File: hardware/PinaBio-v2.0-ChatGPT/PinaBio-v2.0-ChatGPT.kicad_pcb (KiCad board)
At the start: 4 copper layers, 96 x 96 mm, 93 parts, among them J1 USB-C USB2.0 16P, J2 LiPo 1S protected + NTC, J3 AD8232 external module, J4 GSR, J5 RESP_T, J6 RESP_A, J7 GY-30102 external, J8 CJMCU-30205 external, J9 DEBUG UART, SW1 ON/OFF DPDT, SW2 BOOT, SW3 RESET, U1 USBLC6-2SC6, U2 BQ24074RGT, U3 TPS63070RNM, U4 TLV75530PDBVR, U5 ESP32-S3-MINI-1U-N8, U6 ADS122C04IPW, U7 ADS122C04IPW, U8 MCP6004

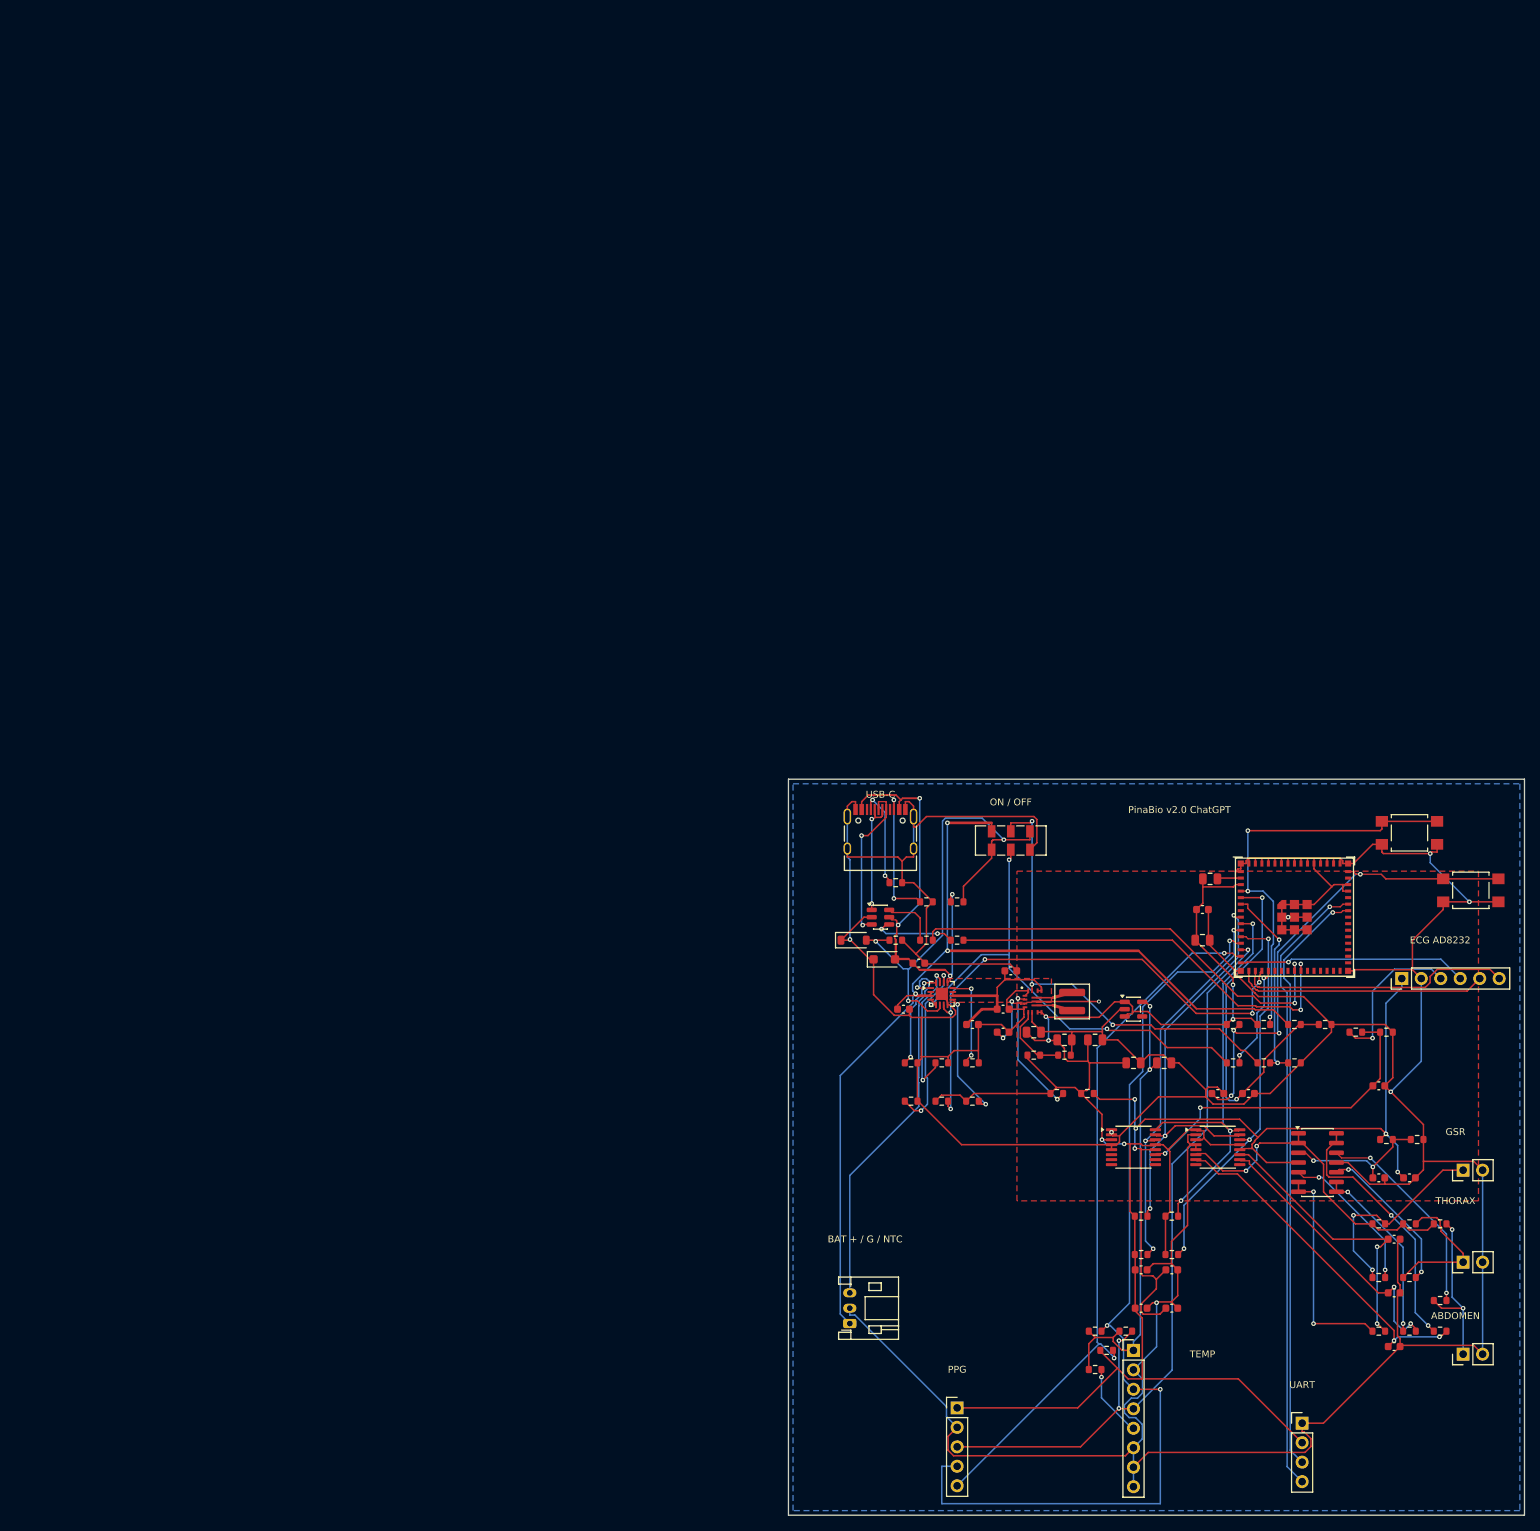
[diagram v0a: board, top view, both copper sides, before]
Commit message: Complete PinaBio Paca v2 ChatGPT KiCad 9 prototype
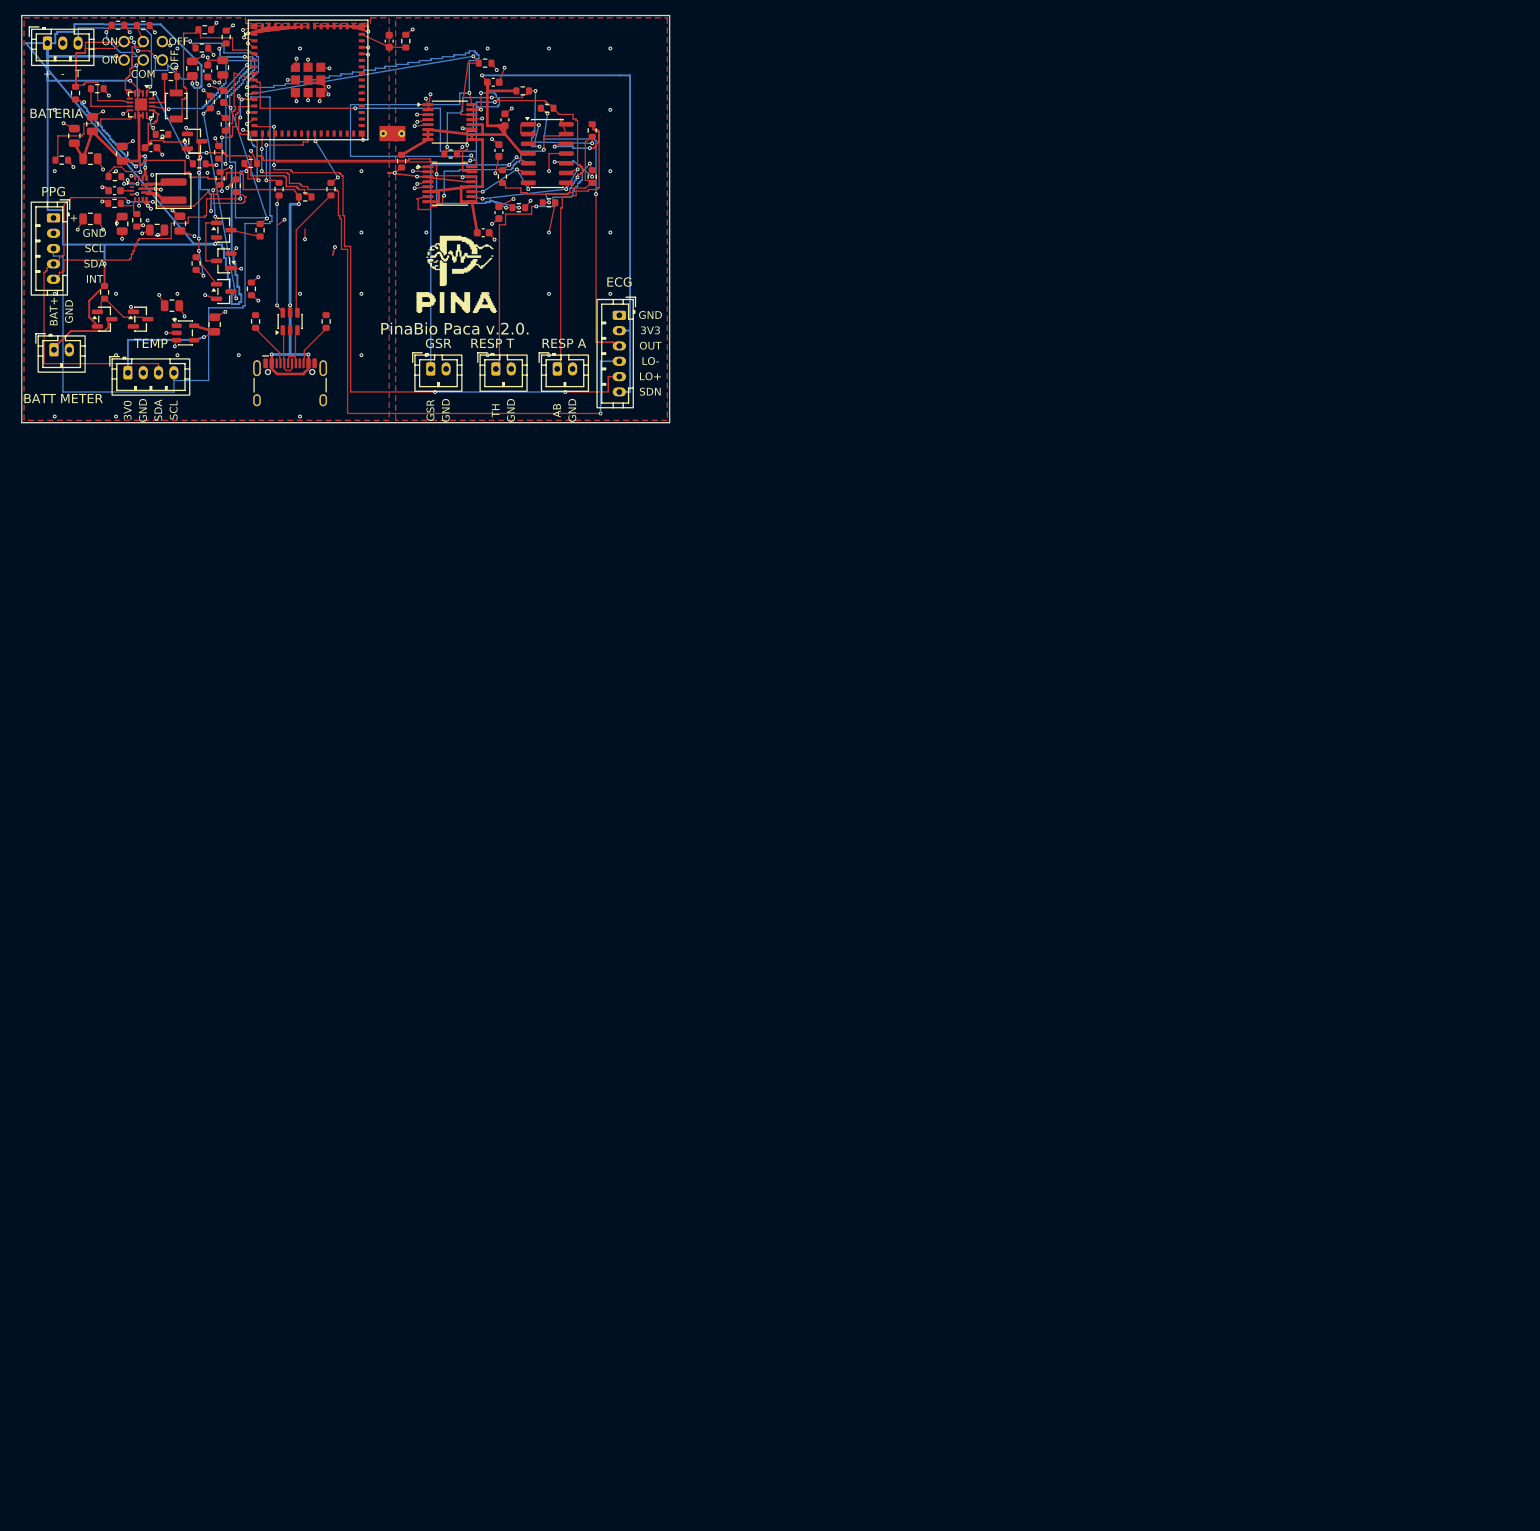
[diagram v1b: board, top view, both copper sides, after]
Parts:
- removed C23: 100nF X7R, Capacitor_SMD:C_0603_1608Metric
- removed C24, C25, C26: 1uF X7R, Capacitor_SMD:C_0603_1608Metric
- removed D2: SMF5.0A, Diode_SMD:D_SOD-123F
- removed R41, R42: 4.7k, Resistor_SMD:R_0603_1608Metric
- removed R43, R44: 10k, Resistor_SMD:R_0603_1608Metric
- removed SW3: RESET, Button_Switch_SMD:SW_SPST_TL3305A
- added NT1: GND_TIE, PinaCursor:GndTie_2mm, F.Cu at (48.3, 15.8)
- added Q1: BSS84, Package_TO_SOT_SMD:SOT-23, F.Cu at (26.3, 28.4)
- added Q2: BSS138, Package_TO_SOT_SMD:SOT-23, F.Cu at (26.3, 32.4)
- added Q3: BSS138, Package_TO_SOT_SMD:SOT-23, F.Cu at (26.3, 36.4)
- added Q4: BSS84, Package_TO_SOT_SMD:SOT-23, F.Cu at (10.8, 40.0)
- added Q5: BSS138, Package_TO_SOT_SMD:SOT-23, F.Cu at (15.5, 40.0)
- C1: value 1uF 16V X7R -> 4.7uF
- C10: value 2.2uF 6.3V X7R -> 10uF
- C11: value 2.2uF 6.3V X7R -> 100nF; footprint Capacitor_SMD:C_0805_2012Metric -> Capacitor_SMD:C_0603_1608Metric
- C12: value 1uF X7R -> 2.2uF; footprint Capacitor_SMD:C_0603_1608Metric -> Capacitor_SMD:C_0805_2012Metric
- C13: value 100nF X7R -> 2.2uF; footprint Capacitor_SMD:C_0603_1608Metric -> Capacitor_SMD:C_0805_2012Metric
- C14: value 10uF 6.3V X7R -> 100nF; footprint Capacitor_SMD:C_0805_2012Metric -> Capacitor_SMD:C_0603_1608Metric
- C15: value 100nF X7R -> 1uF
- C16: value 10uF 6.3V X7R -> 10uF
- C17, C18, C19, C20: value 100nF X7R -> 100nF
- C2: value 4.7uF 10V X7R -> 10uF; footprint Capacitor_SMD:C_0603_1608Metric -> Capacitor_SMD:C_0805_2012Metric
- C21: value 33nF X7R -> 100nF
- C22: value 1uF X7R -> 100nF
- C3, C4, C5: value 10uF 10V X7R -> 10uF; footprint Capacitor_SMD:C_0603_1608Metric -> Capacitor_SMD:C_0805_2012Metric
- C6: value 100nF X7R -> 10uF; footprint Capacitor_SMD:C_0603_1608Metric -> Capacitor_SMD:C_0805_2012Metric
- C7, C8, C9: value 22uF 6.3V X7R -> 22uF
- D1: value BZT52C3V3 -> BZX84-C3V6; footprint Diode_SMD:D_SOD-123 -> Package_TO_SOT_SMD:SOT-23
- J1: value USB-C USB2.0 16P -> USB-C; footprint Connector_USB:USB_C_Receptacle_HRO_TYPE-C-31-M-12 -> Connector_USB:USB_C_Receptacle_HCTL_HC-TYPE-C-16P-01A
- J2: value LiPo 1S protected + NTC -> J_BATT; footprint Connector_JST:JST_PH_S3B-PH-K_1x03_P2.00mm_Horizontal -> Connector_JST:JST_PH_B3B-PH-K_1x03_P2.00mm_Vertical
- J3: value AD8232 external module -> J_ECG; footprint Connector_PinHeader_2.54mm:PinHeader_1x06_P2.54mm_Vertical -> Connector_JST:JST_PH_B6B-PH-K_1x06_P2.00mm_Vertical
- J4: value GSR -> J_PPG; footprint Connector_PinHeader_2.54mm:PinHeader_1x02_P2.54mm_Vertical -> Connector_JST:JST_PH_B5B-PH-K_1x05_P2.00mm_Vertical
- J5: value RESP_T -> J_TEMP; footprint Connector_PinHeader_2.54mm:PinHeader_1x02_P2.54mm_Vertical -> Connector_JST:JST_PH_B4B-PH-K_1x04_P2.00mm_Vertical
- J6: value RESP_A -> J_GSR; footprint Connector_PinHeader_2.54mm:PinHeader_1x02_P2.54mm_Vertical -> Connector_JST:JST_PH_B2B-PH-K_1x02_P2.00mm_Vertical
- J7: value GY-30102 external -> J_RESP_T; footprint Connector_PinHeader_2.54mm:PinHeader_1x05_P2.54mm_Vertical -> Connector_JST:JST_PH_B2B-PH-K_1x02_P2.00mm_Vertical
- J8: value CJMCU-30205 external -> J_RESP_A; footprint Connector_PinHeader_2.54mm:PinHeader_1x08_P2.54mm_Vertical -> Connector_JST:JST_PH_B2B-PH-K_1x02_P2.00mm_Vertical
- J9: value DEBUG UART -> J_BATT_METER; footprint Connector_PinHeader_2.54mm:PinHeader_1x04_P2.54mm_Vertical -> Connector_JST:JST_PH_B2B-PH-K_1x02_P2.00mm_Vertical
- L1: value XAL4020-152MEC 1.5uH -> 1.5uH
- R1, R2: value 5.1k 1% -> 5.1k
- R10: value 46.4k 1% -> 100k
- R11, R12: value 10k -> 100k
- R15: value 10k -> 0
- R16: value 0R -> 1M
- R17: value 10k -> 1M
- R18: value 10k -> 330k
- R19: value 1M 1% -> 100k
- R20: value 330k 1% -> 100k
- R22: value 100k -> 10k
- R23: value 100k -> 4.7k
- R24: value 2.2k -> 4.7k
- R25: value 2.2k -> 10k
- R28: value 33.2k 1% -> 56k 1%
- R29: value 47.5k 1% -> 10k 1%
- R3: value 100k 1% -> 0
- R30: value 56k 1% -> 100k
- R31: value 10k 1% -> 100k
- R32: value 100k 1% -> 100k
- R33: value 100k 1% -> 33.2k 1%
- R34: value 100k 1% -> 47.5k 1%
- R35, R36: value 100k 1% -> 22
- R37: value 100k 1% -> 46.4k 1%
- R38: value 10k 1% -> 10k
- R4: value 150k 1% -> 10.0k
- R40: value 10k 1% -> 1M
- R5: value 22R -> 15.0k
- R6: value 22R -> 2.94k 1%
- R7: value 3.00k 1% -> 2.94k 1%
- R8: value 3.00k 1% -> 2.2k
- R9: value 1.50k 1% -> 100k
- SW1: value ON/OFF DPDT -> DPDT caja; footprint Button_Switch_SMD:SW_DPDT_CK_JS202011JCQN -> PinaCursor:SW_ext_6pad
- SW2: footprint Button_Switch_SMD:SW_SPST_TL3305A -> Button_Switch_SMD:SW_SPST_B3U-1000P
- U2: value BQ24074RGT -> BQ24074
- U3: value TPS63070RNM -> TPS63070; footprint PinaBio-ChatGPT:TPS63070_RNM0015A -> PinaCursor:TPS63070RNM
- U5: footprint PinaBio-ChatGPT:ESP32-S3-MINI-1U -> RF_Module:ESP32-S2-MINI-1U
- U6, U7: value ADS122C04IPW -> ADS122C04
- moved R38 228.6 mm to (23.9, 2.25)
- moved R39 226.3 mm to (12.2, 21.4)
- moved J4 221.9 mm to (4.14, 26.8), turned to -90 degrees
- moved R40 220.7 mm to (10.8, 36.5), turned to 90 degrees
- moved R37 218.7 mm to (25.7, 18.2), turned to 90 degrees
- moved J9 214.7 mm to (4.20, 44.0)
- moved J5 209.3 mm to (13.8, 47.0), turned to 0 degrees
- moved R35 201.8 mm to (33.6, 23.0), turned to 90 degrees
- moved R36 199.9 mm to (40.3, 23.0), turned to 90 degrees
- moved C17 198.2 mm to (24.3, 7.63), turned to 90 degrees
- moved J2 197.1 mm to (3.35, 4.00), turned to 0 degrees
- moved R24 195.5 mm to (23.5, 4.63)
- moved R18 186.8 mm to (26.7, 3.20), turned to 90 degrees
- moved SW2 186.7 mm to (20.1, 12.2), turned to 90 degrees
- moved J6 186.1 mm to (53.3, 46.5), turned to 0 degrees
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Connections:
- net BAT_NTC renamed /TS
- net CC1 renamed /CC1
- net CC2 renamed /CC2
- net TPS_FB renamed /FB
- net TPS_L1 renamed /SW_L1
- net TPS_L2 renamed /SW_L2
- net USB_DN_RAW renamed /USB_DM_C
- net USB_DP_RAW renamed /USB_DP_C
- C1 pad 1: VBUS_RAW -> /VBUS_RAW
- C1 pad 2: GND -> /GND
- C10 pad 1: 3V3_SYS -> /3V3_SYS
- C10 pad 2: GND -> /GND
- C11 pad 1: 3V0_TEMP -> /VAUX
- C11 pad 2: GND -> /GND
- C12 pad 1: ESP_EN -> /3V3_SYS
- C12 pad 2: GND -> /GND
- C13 pad 1: BAT_SENSE -> /3V0_TEMP
- C13 pad 2: GND -> /GND
- C14 pad 1: 3V3_SYS -> /BAT_SENSE
- C14 pad 2: GND -> /GND
- C15 pad 1: 3V3_SYS -> /EN_MOD
- C15 pad 2: GND -> /GND
- C16 pad 1: 3V3_SYS -> /3V3_SYS
- C16 pad 2: GND -> /GND
- C17 pad 1: 3V3_SYS -> /3V3_SYS
- C17 pad 2: GND -> /GND
- C18 pad 1: 3V3_A -> /3V3_A
- C18 pad 2: GND -> /AGND
- C19 pad 1: 3V3_SYS -> /3V3_SYS
- C19 pad 2: GND -> /AGND
- C2 pad 1: BAT_PROT -> /SYS
- C2 pad 2: GND -> /GND
- C20 pad 1: 3V3_A -> /3V3_A
- C20 pad 2: GND -> /AGND
- C21 pad 1: ECG_ADC -> /3V3_SYS
- C21 pad 2: GND -> /AGND
- C22 pad 1: EXC_DIV -> /3V3_A
- C22 pad 2: GND -> /AGND
- C3 pad 1: SYS -> /BAT_PROT
- C3 pad 2: GND -> /GND
- C4 pad 1: SYS -> /SYS
- C4 pad 2: GND -> /GND
- C5 pad 1: SYS -> /SYS
- C5 pad 2: GND -> /GND
- C6 pad 1: TPS_VAUX -> /SYS
- C6 pad 2: GND -> /GND
- C7 pad 1: 3V3_SYS -> /3V3_SYS
- C7 pad 2: GND -> /GND
- C8 pad 1: 3V3_SYS -> /3V3_SYS
- C8 pad 2: GND -> /GND
- C9 pad 1: 3V3_SYS -> /3V3_SYS
- C9 pad 2: GND -> /GND
- D1 pad 1: GND -> /GND
- D1 pad 2: VBUS_MODE -> unconnected-(D1-NC-Pad2)
- J1 pad A1: GND -> /GND
- J1 pad A12: GND -> /GND
- J1 pad A4: VBUS_RAW -> /VBUS
- J1 pad A8: (no net) -> unconnected-(J1-SBU1-PadA8)
- J1 pad A9: VBUS_RAW -> /VBUS
- J1 pad B1: GND -> /GND
- J1 pad B12: GND -> /GND
- J1 pad B4: VBUS_RAW -> /VBUS
- J1 pad B8: (no net) -> unconnected-(J1-SBU2-PadB8)
- J1 pad B9: VBUS_RAW -> /VBUS
- J1 pad S1: GND -> /GND
- J2 pad 1: BAT_PROT -> /BAT_PROT
- J2 pad 2: GND -> /GND
- J3 pad 1: 3V3_A -> /AGND
- J3 pad 2: GND -> /3V3_A
- J3 pad 3: ECG_OUT -> /ECG_OUT
- J3 pad 4: ECG_LOP -> /LO_N
- J3 pad 5: ECG_LON -> /LO_P
- J3 pad 6: ECG_SDN -> /3V3_A
- J4 pad 1: GSR_ELECTRODE -> /3V3_SYS
- J4 pad 2: GND -> /GND
- J5 pad 1: RESP_T_ELECTRODE -> /3V0_TEMP
- J5 pad 2: GND -> /GND
- J6 pad 1: RESP_A_ELECTRODE -> /SNS_GSR
- J6 pad 2: GND -> /AGND
- J7 pad 1: 3V3_SYS -> /SNS_TH
- J7 pad 2: GND -> /AGND
- J8 pad 1: 3V0_TEMP -> /SNS_AB
- J8 pad 2: GND -> /AGND
- J9 pad 1: GND -> /BAT_METER
- J9 pad 2: 3V3_SYS -> /GND
- R1 pad 2: GND -> /GND
- R10 pad 1: BQ_TMR -> /PGOOD
- R10 pad 2: GND -> /3V3_SYS
- R11 pad 1: 3V3_SYS -> /EN2_CE
- R11 pad 2: USB_VALID_N -> /GND
- R12 pad 1: 3V3_SYS -> /TPS_EN
- R12 pad 2: BQ_CHG -> /GND
- R13 pad 1: 3V3_SYS -> /3V3_SYS
- R14 pad 2: GND -> /GND
- R15 pad 1: 3V3_SYS -> /3V3_SYS
- R15 pad 2: TPS_PG -> /3V3_A
- R16 pad 1: 3V3_SYS -> /Q1G
- R16 pad 2: 3V3_A -> /BAT_PROT
- R17 pad 1: 3V3_SYS -> /DIV_IN
- R17 pad 2: ESP_EN -> /BAT_SENSE
- R18 pad 1: 3V3_SYS -> /BAT_SENSE
- R18 pad 2: BOOT_IO0 -> /GND
- R19 pad 1: BAT_PROT -> /3V3_SYS
- R19 pad 2: BAT_SENSE -> /GND
- R2 pad 2: GND -> /GND
- R20 pad 1: BAT_SENSE -> /VLOG
- R20 pad 2: GND -> /VBUS_G
- R21 pad 1: BQ_EN2_CE -> /VBUS_N
- R21 pad 2: BQ_MODE_SENSE -> /3V3_SYS
- R22 pad 1: TPS_EN -> /EN_MOD
- R22 pad 2: SW_ON_SENSE -> /3V3_SYS
- R23 pad 1: SW_ON_SENSE -> /SDA_ADC
- R23 pad 2: GND -> /3V3_SYS
- R24 pad 1: 3V3_SYS -> /SCL_ADC
- R24 pad 2: ADC_SDA -> /3V3_SYS
- R25 pad 1: 3V3_SYS -> /PPG_INT
- R25 pad 2: ADC_SCL -> /3V3_SYS
- R26 pad 1: 3V3_SYS -> /DRDY_ECG
- R26 pad 2: ADC_DRDY_ECG -> /3V3_SYS
- R27 pad 1: 3V3_SYS -> /DRDY_SLOW
- R27 pad 2: ADC_DRDY_SLOW -> /3V3_SYS
- R28 pad 1: ECG_OUT -> /3V3_A
- R28 pad 2: ECG_ADC -> /DIV_EXC
- R29 pad 1: ECG_ADC -> /DIV_EXC
- R29 pad 2: GND -> /AGND
- R3 pad 1: VBUS_RAW -> /VBUS
- R3 pad 2: VBUS_MODE -> /VBUS_RAW
- R30 pad 1: 3V3_A -> /0V5_EXC
- R30 pad 2: EXC_DIV -> /SNS_GSR
- R31 pad 1: EXC_DIV -> /0V5_EXC
- R31 pad 2: GND -> /SNS_TH
- R32 pad 1: 0V5_EXC -> /0V5_EXC
- R32 pad 2: GSR_ELECTRODE -> /SNS_AB
- R33 pad 1: 0V5_EXC -> /ECG_OUT
- R33 pad 2: RESP_T_ELECTRODE -> /ECG_DIV
- R34 pad 1: 0V5_EXC -> /ECG_DIV
- R34 pad 2: RESP_A_ELECTRODE -> /AGND
- R35 pad 1: GSR_ELECTRODE -> /USB_DM
- R35 pad 2: GSR_SENSE -> /USB_DM_IO
- R36 pad 1: RESP_T_ELECTRODE -> /USB_DP
- R36 pad 2: RESP_T_SENSE -> /USB_DP_IO
- R37 pad 1: RESP_A_ELECTRODE -> /TMR
- R37 pad 2: RESP_A_SENSE -> /GND
- R38 pad 1: GSR_BUF -> /BOOT
- R38 pad 2: GSR_ADC -> /3V3_SYS
- R39 pad 1: RESP_T_BUF -> /TPS_EN
- R39 pad 2: RESP_T_ADC -> /TPS_EN_IC
- R4 pad 1: VBUS_MODE -> /VBUS
- R4 pad 2: GND -> /VLOG
- R40 pad 1: RESP_A_BUF -> /METER_GATE
- R40 pad 2: RESP_A_ADC -> /BAT_PROT
- R5 pad 1: USB_DN_ESD -> /VLOG
- R5 pad 2: USB_DN_MCU -> /GND
- R6 pad 1: USB_DP_ESD -> /ISET
- R6 pad 2: USB_DP_MCU -> /GND
- R7 pad 1: BQ_ISET -> /ITERM
- R7 pad 2: GND -> /GND
- R8 pad 1: BQ_ITERM -> /ILIM
- R8 pad 2: GND -> /GND
- R9 pad 1: BQ_ILIM -> /CHG
- R9 pad 2: GND -> /3V3_SYS
- SW1 pad 1: BAT_PROT -> /VLOG
- SW1 pad 2: TPS_EN -> /EN2_CE
- SW1 pad 3: VBUS_MODE -> /GND
- SW1 pad 4: VBUS_MODE -> /BAT_PROT
- SW1 pad 5: BQ_EN2_CE -> /TPS_EN
- SW1 pad 6: GND -> /VLOG
- SW2 pad 1: BOOT_IO0 -> /BOOT
- SW2 pad 2: GND -> /GND
- U1 pad 2: GND -> /GND
- U1 pad 4: USB_DP_ESD -> /USB_DP
- U1 pad 5: VBUS_RAW -> /VBUS
- U1 pad 6: USB_DN_ESD -> /USB_DM
- U2 pad 10: SYS -> /SYS
- U2 pad 11: SYS -> /SYS
- U2 pad 12: BQ_ILIM -> /ILIM
- U2 pad 13: VBUS_RAW -> /VBUS_RAW
- U2 pad 14: BQ_TMR -> /TMR
- U2 pad 15: BQ_ITERM -> /ITERM
- U2 pad 16: BQ_ISET -> /ISET
- U2 pad 17: GND -> /GND
- U2 pad 2: BAT_PROT -> /BAT_PROT
- U2 pad 3: BAT_PROT -> /BAT_PROT
- U2 pad 4: BQ_EN2_CE -> /EN2_CE
- U2 pad 5: BQ_EN2_CE -> /EN2_CE
- U2 pad 6: VBUS_MODE -> /VLOG
- U2 pad 7: USB_VALID_N -> /PGOOD
- U2 pad 8: GND -> /GND
- U2 pad 9: BQ_CHG -> /CHG
- U3 pad 1: GND -> /GND
- U3 pad 10: GND -> /GND
- U3 pad 12: SYS -> /SYS
- U3 pad 13: SYS -> /SYS
- U3 pad 14: TPS_EN -> /TPS_EN_IC
- U3 pad 15: GND -> /GND
- U3 pad 2: TPS_PG -> unconnected-(U3-PG-Pad2)
- U3 pad 3: TPS_VAUX -> /VAUX
- U3 pad 4: GND -> /GND
- U3 pad 6: GND -> /GND
- U3 pad 7: 3V3_SYS -> /3V3_SYS
- U3 pad 8: 3V3_SYS -> /3V3_SYS
- U4 pad 1: 3V3_SYS -> /3V3_SYS
- U4 pad 2: GND -> /GND
- U4 pad 3: 3V3_SYS -> /3V3_SYS
- U4 pad 4: (no net) -> unconnected-(U4-NC-Pad4)
- U4 pad 5: 3V0_TEMP -> /3V0_TEMP
- U5 pad 1: GND -> /GND
- U5 pad 10: ADC_DRDY_ECG -> /DRDY_ECG
- U5 pad 11: ADC_DRDY_SLOW -> /DRDY_SLOW
- U5 pad 12: EXT_SDA -> /SDA_MOD
- U5 pad 13: EXT_SCL -> /SCL_MOD
- U5 pad 14: PPG_INT -> /PPG_INT
- U5 pad 15: ECG_LOP -> /LO_P
- U5 pad 16: ECG_LON -> /LO_N
- U5 pad 17: ECG_SDN -> unconnected-(U5-IO13-Pad17)
- U5 pad 18: USB_VALID_N -> unconnected-(U5-IO14-Pad18)
- U5 pad 19: BQ_MODE_SENSE -> unconnected-(U5-IO15-Pad19)
- U5 pad 2: GND -> /GND
- U5 pad 20: (no net) -> unconnected-(U5-IO16-Pad20)
- U5 pad 21: (no net) -> unconnected-(U5-IO17-Pad21)
- U5 pad 22: (no net) -> unconnected-(U5-IO18-Pad22)
- U5 pad 23: USB_DN_MCU -> /USB_DM_IO
- U5 pad 24: USB_DP_MCU -> /USB_DP_IO
- U5 pad 25: (no net) -> unconnected-(U5-IO21-Pad25)
- U5 pad 26: (no net) -> unconnected-(U5-IO26-Pad26)
- U5 pad 27: (no net) -> unconnected-(U5-IO47-Pad27)
- U5 pad 28: (no net) -> unconnected-(U5-IO33-Pad28)
- U5 pad 29: (no net) -> unconnected-(U5-IO34-Pad29)
- U5 pad 3: 3V3_SYS -> /3V3_SYS
- U5 pad 30: (no net) -> unconnected-(U5-IO48-Pad30)
- U5 pad 31: (no net) -> unconnected-(U5-IO35-Pad31)
- U5 pad 32: (no net) -> unconnected-(U5-IO36-Pad32)
- U5 pad 33: (no net) -> unconnected-(U5-IO37-Pad33)
- U5 pad 34: (no net) -> unconnected-(U5-IO38-Pad34)
- U5 pad 35: (no net) -> unconnected-(U5-IO39-Pad35)
- U5 pad 36: (no net) -> unconnected-(U5-IO40-Pad36)
- U5 pad 37: (no net) -> unconnected-(U5-IO41-Pad37)
- U5 pad 38: (no net) -> unconnected-(U5-IO42-Pad38)
- U5 pad 39: UART_TX -> unconnected-(U5-TXD0-Pad39)
- U5 pad 4: BOOT_IO0 -> /BOOT
- U5 pad 40: UART_RX -> unconnected-(U5-RXD0-Pad40)
- U5 pad 41: (no net) -> unconnected-(U5-IO45-Pad41)
- U5 pad 42: GND -> /GND
- U5 pad 43: GND -> /GND
- U5 pad 44: (no net) -> unconnected-(U5-IO46-Pad44)
- U5 pad 45: ESP_EN -> /EN_MOD
- U5 pad 46: GND -> /GND
- U5 pad 47: GND -> /GND
- U5 pad 48: GND -> /GND
- U5 pad 49: GND -> /GND
- U5 pad 5: BAT_SENSE -> /BAT_SENSE
- U5 pad 50: GND -> /GND
- U5 pad 51: GND -> /GND
- U5 pad 52: GND -> /GND
- U5 pad 53: GND -> /GND
- U5 pad 54: GND -> /GND
- U5 pad 55: GND -> /GND
- U5 pad 56: GND -> /GND
- U5 pad 57: GND -> /GND
- U5 pad 58: GND -> /GND
- U5 pad 59: GND -> /GND
- U5 pad 6: SW_ON_SENSE -> /VBUS_N
- U5 pad 60: GND -> /GND
- U5 pad 61: GND -> /GND
- U5 pad 62: GND -> /GND
- U5 pad 63: GND -> /GND
- U5 pad 64: GND -> /GND
- U5 pad 65: GND -> /GND
- U5 pad 7: (no net) -> unconnected-(U5-IO3-Pad7)
- U5 pad 8: ADC_SDA -> /SDA_ADC
- U5 pad 9: ADC_SCL -> /SCL_ADC
- U6 pad 1: GND -> /AGND
- U6 pad 10: (no net) -> /3V3_A
- U6 pad 11: ECG_ADC -> /ECG_DIV
- U6 pad 12: 3V3_A -> /3V3_A
- U6 pad 13: 3V3_SYS -> /3V3_SYS
- U6 pad 14: ADC_DRDY_ECG -> /DRDY_ECG
- U6 pad 15: ADC_SDA -> /SDA_ADC
- U6 pad 16: ADC_SCL -> /SCL_ADC
- U6 pad 2: GND -> /AGND
- U6 pad 3: 3V3_SYS -> /3V3_SYS
- U6 pad 4: GND -> /AGND
- U6 pad 5: GND -> /AGND
- U6 pad 6: (no net) -> /3V3_A
- U6 pad 7: (no net) -> /3V3_A
- U6 pad 8: (no net) -> /3V3_A
- U6 pad 9: (no net) -> /3V3_A
- U7 pad 1: 3V3_SYS -> /3V3_SYS
- U7 pad 10: RESP_T_ADC -> /OUT_TH
- U7 pad 11: GSR_ADC -> /OUT_GSR
- U7 pad 12: 3V3_A -> /3V3_A
- U7 pad 13: 3V3_SYS -> /3V3_SYS
- U7 pad 14: ADC_DRDY_SLOW -> /DRDY_SLOW
- U7 pad 15: ADC_SDA -> /SDA_ADC
- U7 pad 16: ADC_SCL -> /SCL_ADC
- U7 pad 2: GND -> /AGND
- U7 pad 3: 3V3_SYS -> /3V3_SYS
- U7 pad 4: GND -> /AGND
- U7 pad 5: GND -> /AGND
- U7 pad 6: 0V5_EXC -> /3V3_A
- U7 pad 7: RESP_A_ADC -> /OUT_AB
- U7 pad 8: (no net) -> /3V3_A
- U7 pad 9: (no net) -> /3V3_A
- U8 pad 1: 0V5_EXC -> /0V5_EXC
- U8 pad 10: RESP_T_SENSE -> /SNS_TH
- U8 pad 11: GND -> /AGND
- U8 pad 12: RESP_A_SENSE -> /SNS_AB
- U8 pad 13: RESP_A_BUF -> /OUT_AB
- U8 pad 14: RESP_A_BUF -> /OUT_AB
- U8 pad 2: 0V5_EXC -> /0V5_EXC
- U8 pad 3: EXC_DIV -> /DIV_EXC
- U8 pad 4: 3V3_A -> /3V3_A
- U8 pad 5: GSR_SENSE -> /SNS_GSR
- U8 pad 6: GSR_BUF -> /OUT_GSR
- U8 pad 7: GSR_BUF -> /OUT_GSR
- U8 pad 8: RESP_T_BUF -> /OUT_TH
- U8 pad 9: RESP_T_BUF -> /OUT_TH
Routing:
- net GND: track 691.3 -> 0.00 mm, vias 8 -> 0
- net 3V3_SYS: track 242.4 -> 0.00 mm, vias 6 -> 0
- net /BAT_PROT: track 0.00 -> 199.6 mm, vias 0 -> 6
- net /GND: track 0.00 -> 142.7 mm, vias 0 -> 79
- net BAT_PROT: track 133.5 -> 0.00 mm, vias 3 -> 0
- net /3V3_A: track 0.00 -> 132.9 mm, vias 0 -> 1
- net EXT_SDA: track 125.9 -> 0.00 mm, vias 3 -> 0
- net 3V3_A: track 118.0 -> 0.00 mm, vias 5 -> 0
- net /SCL_ADC: track 0.00 -> 103.5 mm, vias 0 -> 4
- net EXT_SCL: track 103.2 -> 0.00 mm, vias 3 -> 0
- net /DRDY_SLOW: track 0.00 -> 99.2 mm, vias 0 -> 7
- net /VLOG: track 0.00 -> 96.6 mm, vias 0 -> 11
- net PPG_INT: track 92.7 -> 0.00 mm, vias 2 -> 0
- net /SCL_MOD: track 0.00 -> 92.5 mm, vias 0 -> 1
- net /LO_N: track 0.00 -> 90.0 mm, vias 0 -> 3
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- added copper zone on In2.Cu, net /3V3_SYS
- added copper zone on F.Cu, net /AGND
- added copper zone on In1.Cu, net /AGND
- added copper zone on F.Cu, net /GND
- added copper zone on In1.Cu, net /GND
- removed copper zone on F.Cu, net 3V3_SYS
- removed copper zone on In2.Cu, net 3V3_SYS
- removed copper zone on B.Cu, net GND
- removed copper zone on In1.Cu, net GND
- removed copper zone on F.Cu, net SYS
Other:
- board size 96 x 96 mm -> 84.5 x 53.1 mm
- board text added: "+"
- board text added: "-"
- board text added: "3V0"
- board text added: "3V3"
- board text added: "AB"
- board text added: "BAT+"
- board text added: "BATERIA"
- board text added: "BATT METER"
- board text added: "ECG"
- board text added: "GND"
- board text added: "INT"
- board text added: "LO+"
- board text added: "LO-"
- board text added: "OUT"
- board text added: "PinaBio Paca v.2.0."
- board text added: "RESP A"
- board text added: "RESP T"
- board text added: "SCL"
- board text added: "SDA"
- board text added: "SDN"
- board text added: "T"
- board text added: "TH"
- board text removed: "ABDOMEN"
- board text removed: "BAT + / G / NTC"
- board text removed: "ECG AD8232"
- board text removed: "ON / OFF"
- board text removed: "PinaBio v2.0 ChatGPT"
- board text removed: "THORAX"
- board text removed: "UART"
- board text removed: "USB-C"
